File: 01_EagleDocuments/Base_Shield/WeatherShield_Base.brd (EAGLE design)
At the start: 67.3 x 58.4 mm, 74 parts, among them Q1 BSS138, Q2 BSS138, U1 DS3231SN, U2 LT3652, U3 TMP100MDBVREP, U4 ADS1015IDGST

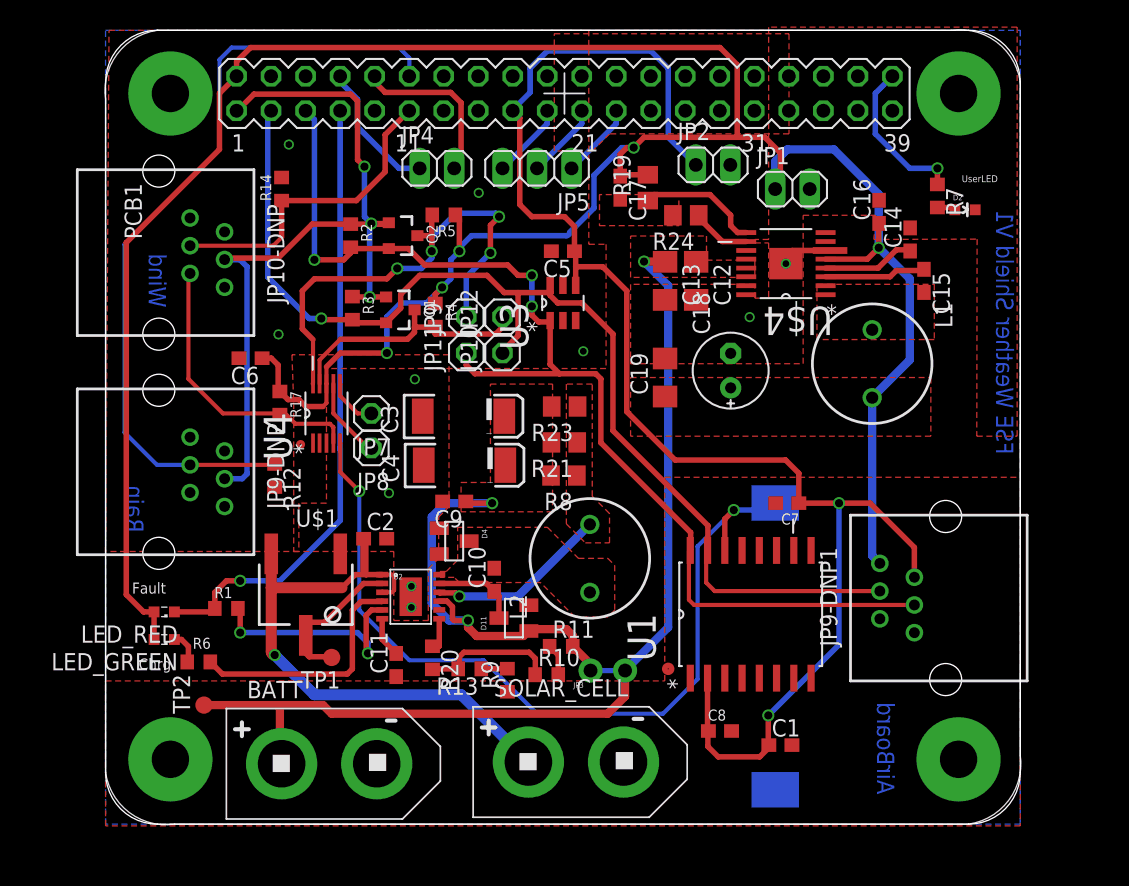
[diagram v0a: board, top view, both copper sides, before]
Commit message: WeatherShield_v1
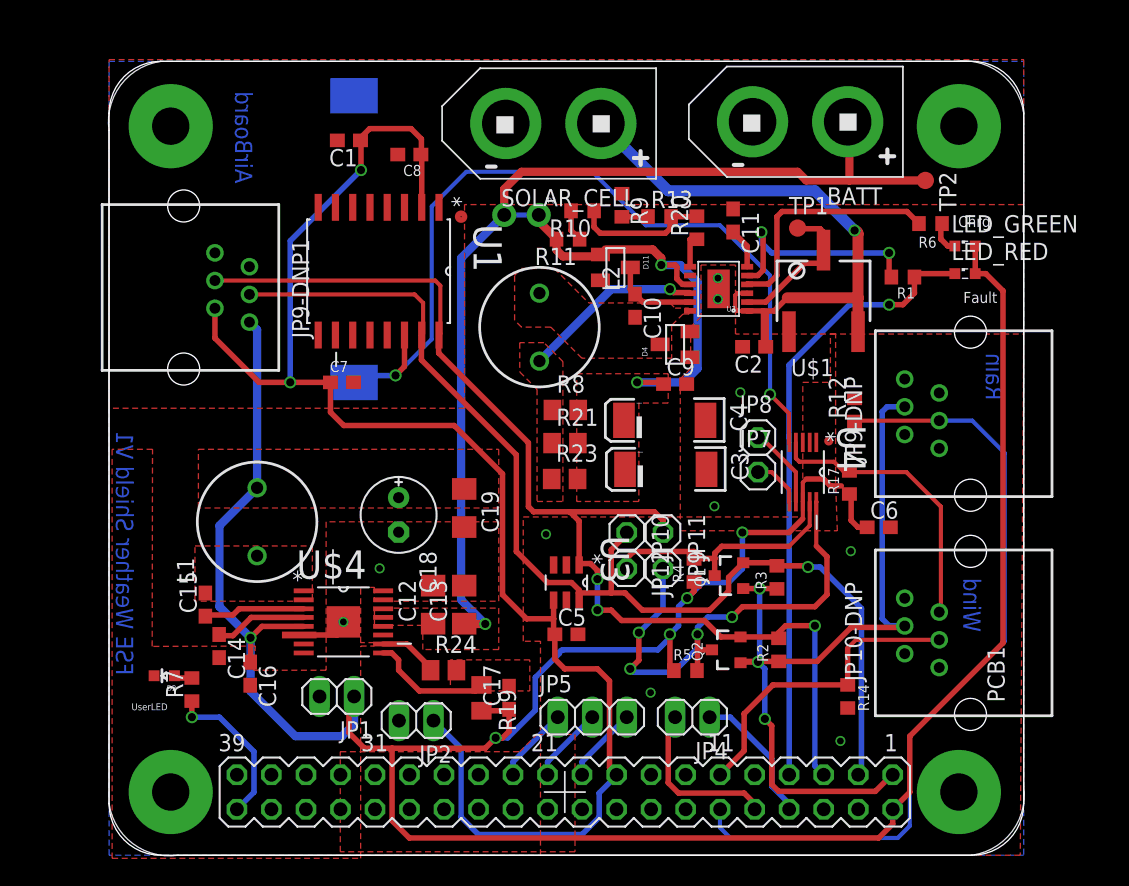
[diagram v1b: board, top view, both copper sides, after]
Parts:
- R17: value 10k -> 20k
- moved PCB1 87.8 mm to (67.6, 58.8), turned to 180 degrees
- moved JP10-DNP 82.2 mm to (69.6, 10.6), turned to 90 degrees
- moved JP9-DNP1 76.6 mm to (-0.25, 48.3), turned to 270 degrees
- moved JP9-DNP 72.2 mm to (69.6, 26.8), turned to 90 degrees
- moved D2 68.2 mm to (4.32, 13.6), turned to 90 degrees
- moved R7 65.8 mm to (6.35, 12.6), turned to 90 degrees
- moved LED_GREEN 65.7 mm to (63.2, 45.2), turned to 0 degrees
- moved TP2 65.6 mm to (60.3, 50.0), turned to 270 degrees
- moved LED_RED 64.0 mm to (63.2, 43.2), turned to 0 degrees
- moved BATT 63.0 mm to (54.6, 54.4), turned to 180 degrees
- moved R6 62.8 mm to (60.7, 46.9), turned to 180 degrees
- moved C14 59.0 mm to (8.36, 15.8), turned to 270 degrees
- moved C15 58.0 mm to (7.34, 18.8), turned to 90 degrees
- moved C16 57.4 mm to (10.6, 13.7), turned to 270 degrees
- moved R14 55.9 mm to (54.6, 12.1), turned to 270 degrees
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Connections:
- net 3.3V: now also R17.1
- net 5V: no longer R17.1
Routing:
- net 5V: track 204.2 -> 203.1 mm

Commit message: WeatherShield_v1
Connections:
- new net N$5: U3.5
- net GND: no longer U3.5
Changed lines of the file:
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@@
 <contactref element="JP1" pad="2"/>
 <contactref element="U3" pad="2"/>
-<contactref element="U3" pad="5"/>
-<contactref element="U3" pad="3"/>
 <polygon width="0.254" layer="1">
 <vertex x="30.734" y="25.273"/>
@@
 <via x="46.7106" y="34.4424" extent="1-16" drill="0.5" diameter="0.254"/>
 <via x="40.1066" y="12.3444" extent="1-16" drill="0.5" diameter="0.254"/>
+<contactref element="U3" pad="3"/>
 </signal>
 <signal name="FAULT_PIN">
@@
 <wire x1="61.468" y1="46.775" x2="61.556" y2="46.863" width="0.4064" layer="1"/>
 </signal>
+<signal name="N$5">
+<contactref element="U3" pad="5"/>
+</signal>
 </signals>
